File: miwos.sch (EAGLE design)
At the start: 44 parts, among them J1 614004190021, U1 PEC16, U3 PEC16

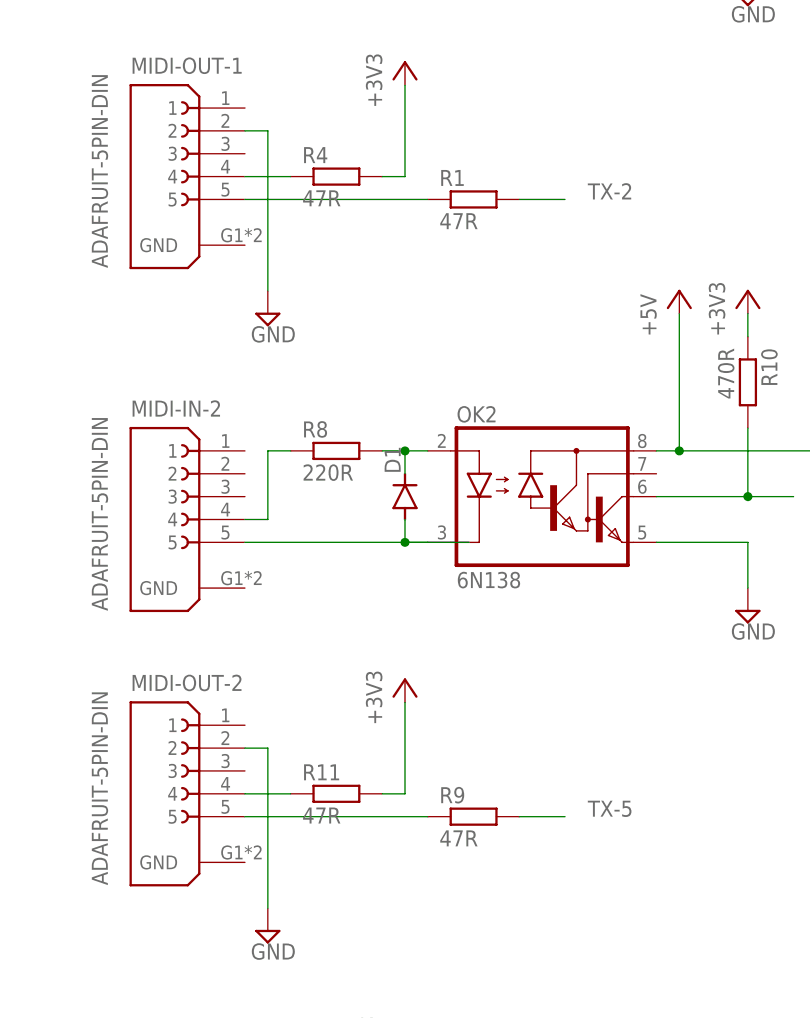
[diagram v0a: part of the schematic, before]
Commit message: Use lorenz's version
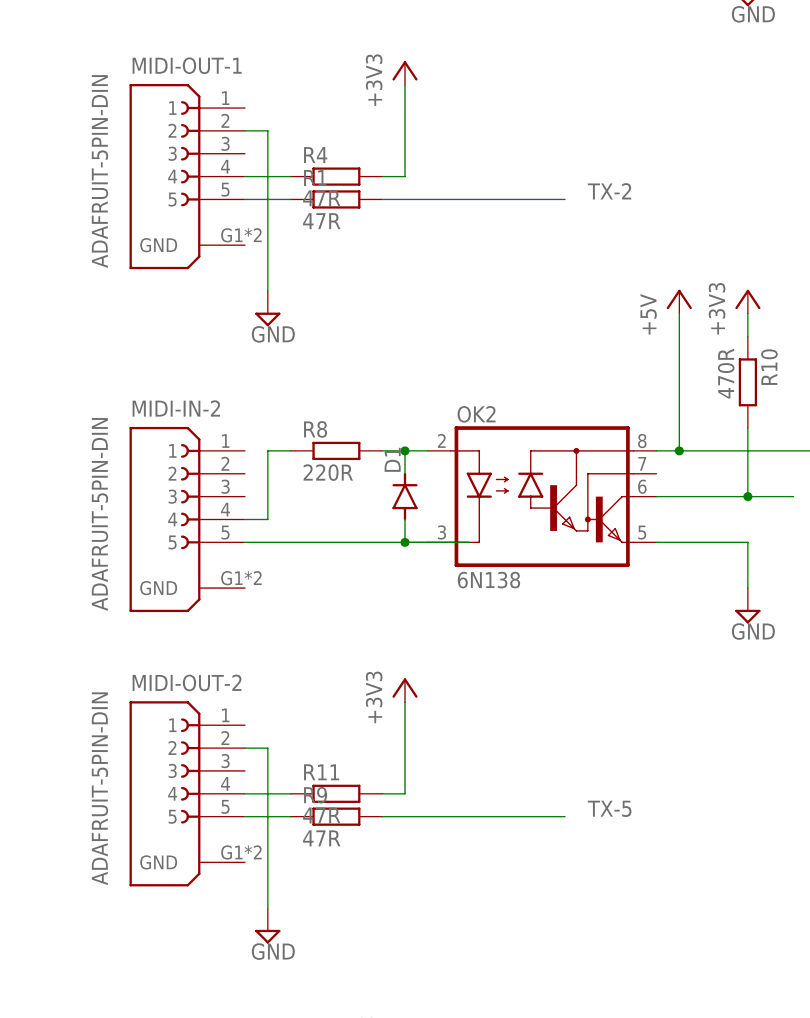
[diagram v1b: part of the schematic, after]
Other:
- moved on the sheet: R1, R9
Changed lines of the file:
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@@
 <attribute name="VALUE" x="131.8514" y="134.62" size="1.778" layer="96" rot="R90"/>
 </instance>
-<instance part="R1" gate="G$1" x="137.16" y="96.52" smashed="yes">
-<attribute name="NAME" x="133.35" y="98.0186" size="1.778" layer="95"/>
-<attribute name="VALUE" x="133.35" y="93.218" size="1.778" layer="96"/>
+<instance part="R1" gate="G$1" x="121.92" y="96.52" smashed="yes">
+<attribute name="NAME" x="118.11" y="98.0186" size="1.778" layer="95"/>
+<attribute name="VALUE" x="118.11" y="93.218" size="1.778" layer="96"/>
 </instance>
 <instance part="P+2" gate="1" x="160.02" y="154.94" smashed="yes">
@@
 <attribute name="VALUE" x="131.8514" y="66.04" size="1.778" layer="96" rot="R90"/>
 </instance>
-<instance part="R9" gate="G$1" x="137.16" y="27.94" smashed="yes">
-<attribute name="NAME" x="133.35" y="29.4386" size="1.778" layer="95"/>
-<attribute name="VALUE" x="133.35" y="24.638" size="1.778" layer="96"/>
+<instance part="R9" gate="G$1" x="121.92" y="27.94" smashed="yes">
+<attribute name="NAME" x="118.11" y="29.4386" size="1.778" layer="95"/>
+<attribute name="VALUE" x="118.11" y="24.638" size="1.778" layer="96"/>
 </instance>
 <instance part="P+3" gate="1" x="160.02" y="86.36" smashed="yes">
@@
 <pinref part="MIDI-OUT-1" gate="G$1" pin="5"/>
 <pinref part="R1" gate="G$1" pin="1"/>
-<wire x1="111.76" y1="96.52" x2="132.08" y2="96.52" width="0.1524" layer="91"/>
+<wire x1="111.76" y1="96.52" x2="116.84" y2="96.52" width="0.1524" layer="91"/>
 </segment>
 </net>
@@
 <pinref part="MIDI-OUT-2" gate="G$1" pin="5"/>
 <pinref part="R9" gate="G$1" pin="1"/>
-<wire x1="111.76" y1="27.94" x2="132.08" y2="27.94" width="0.1524" layer="91"/>
+<wire x1="111.76" y1="27.94" x2="116.84" y2="27.94" width="0.1524" layer="91"/>
 </segment>
 </net>
@@
 <segment>
 <pinref part="R1" gate="G$1" pin="2"/>
-<wire x1="142.24" y1="96.52" x2="147.32" y2="96.52" width="0.1524" layer="91"/>
+<wire x1="127" y1="96.52" x2="147.32" y2="96.52" width="0.1524" layer="91"/>
 <label x="149.86" y="96.52" size="1.778" layer="95"/>
 </segment>
@@
 <segment>
 <pinref part="R9" gate="G$1" pin="2"/>
-<wire x1="142.24" y1="27.94" x2="147.32" y2="27.94" width="0.1524" layer="91"/>
+<wire x1="127" y1="27.94" x2="147.32" y2="27.94" width="0.1524" layer="91"/>
 <label x="149.86" y="27.94" size="1.778" layer="95"/>
 </segment>
